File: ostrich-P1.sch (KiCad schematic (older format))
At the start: 25 parts

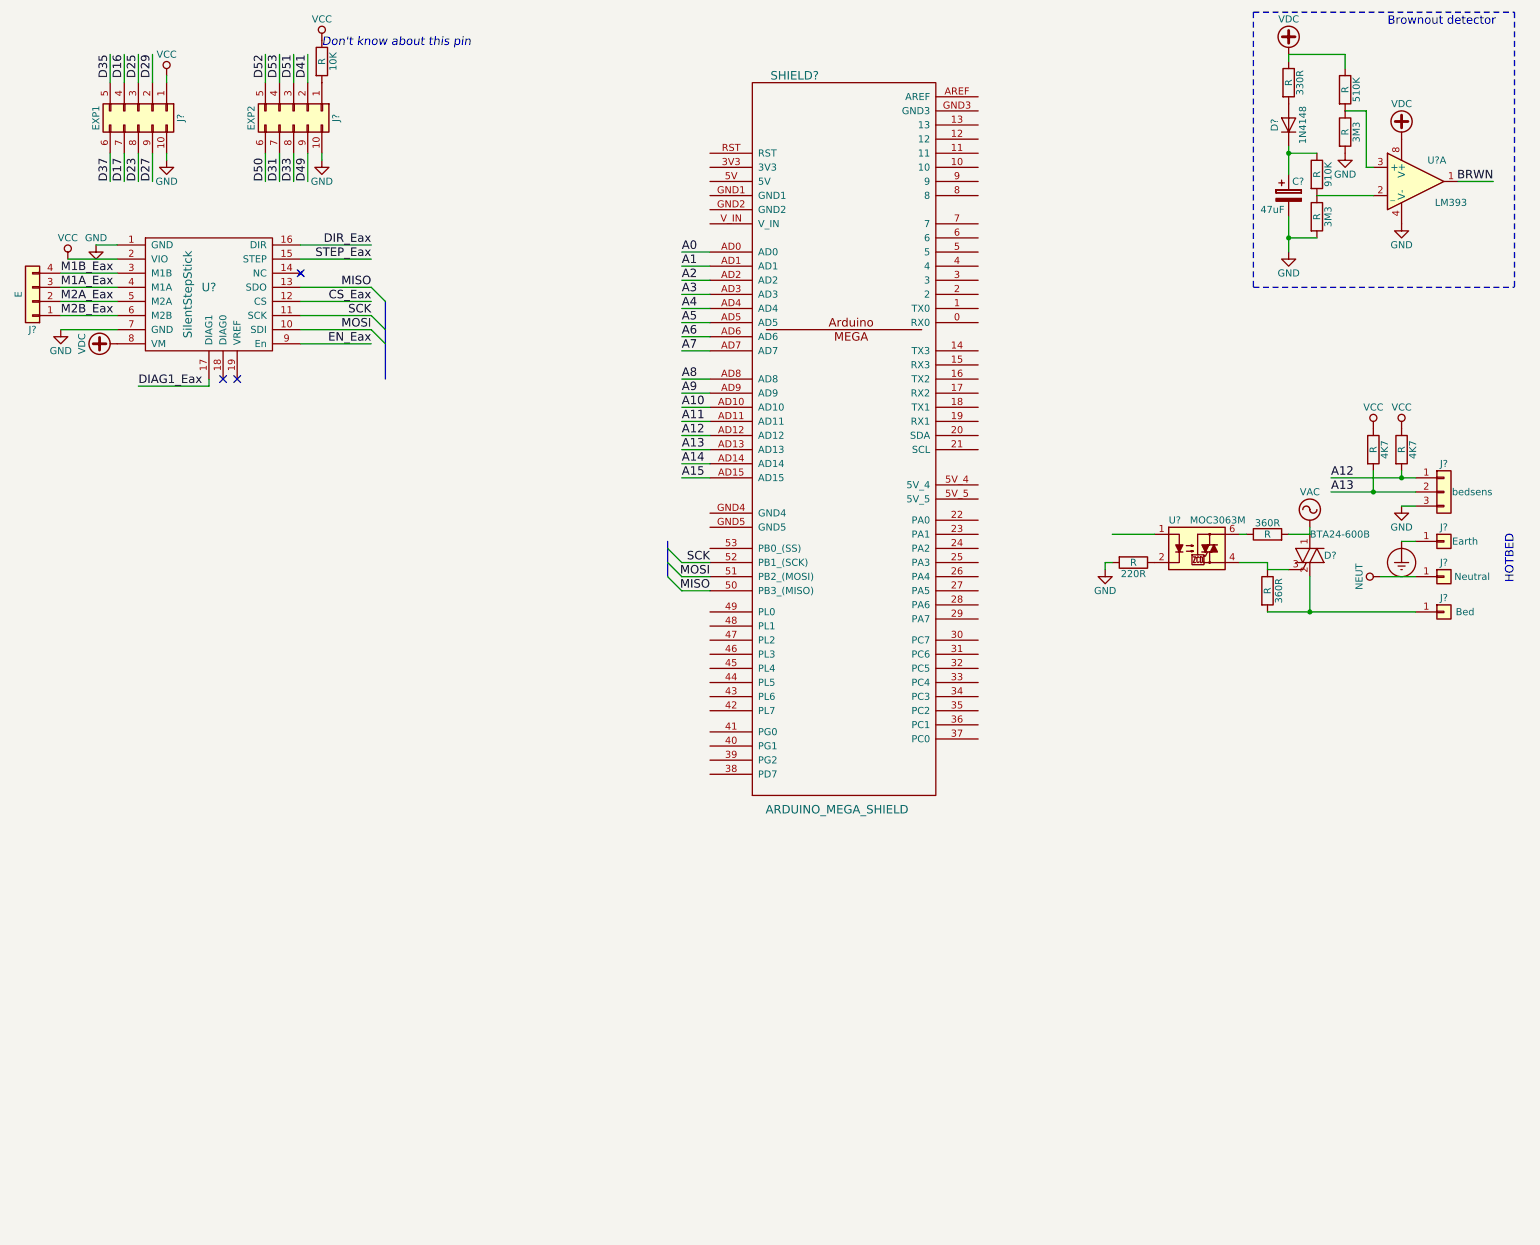
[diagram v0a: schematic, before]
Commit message: 3.3V reg and ESP12
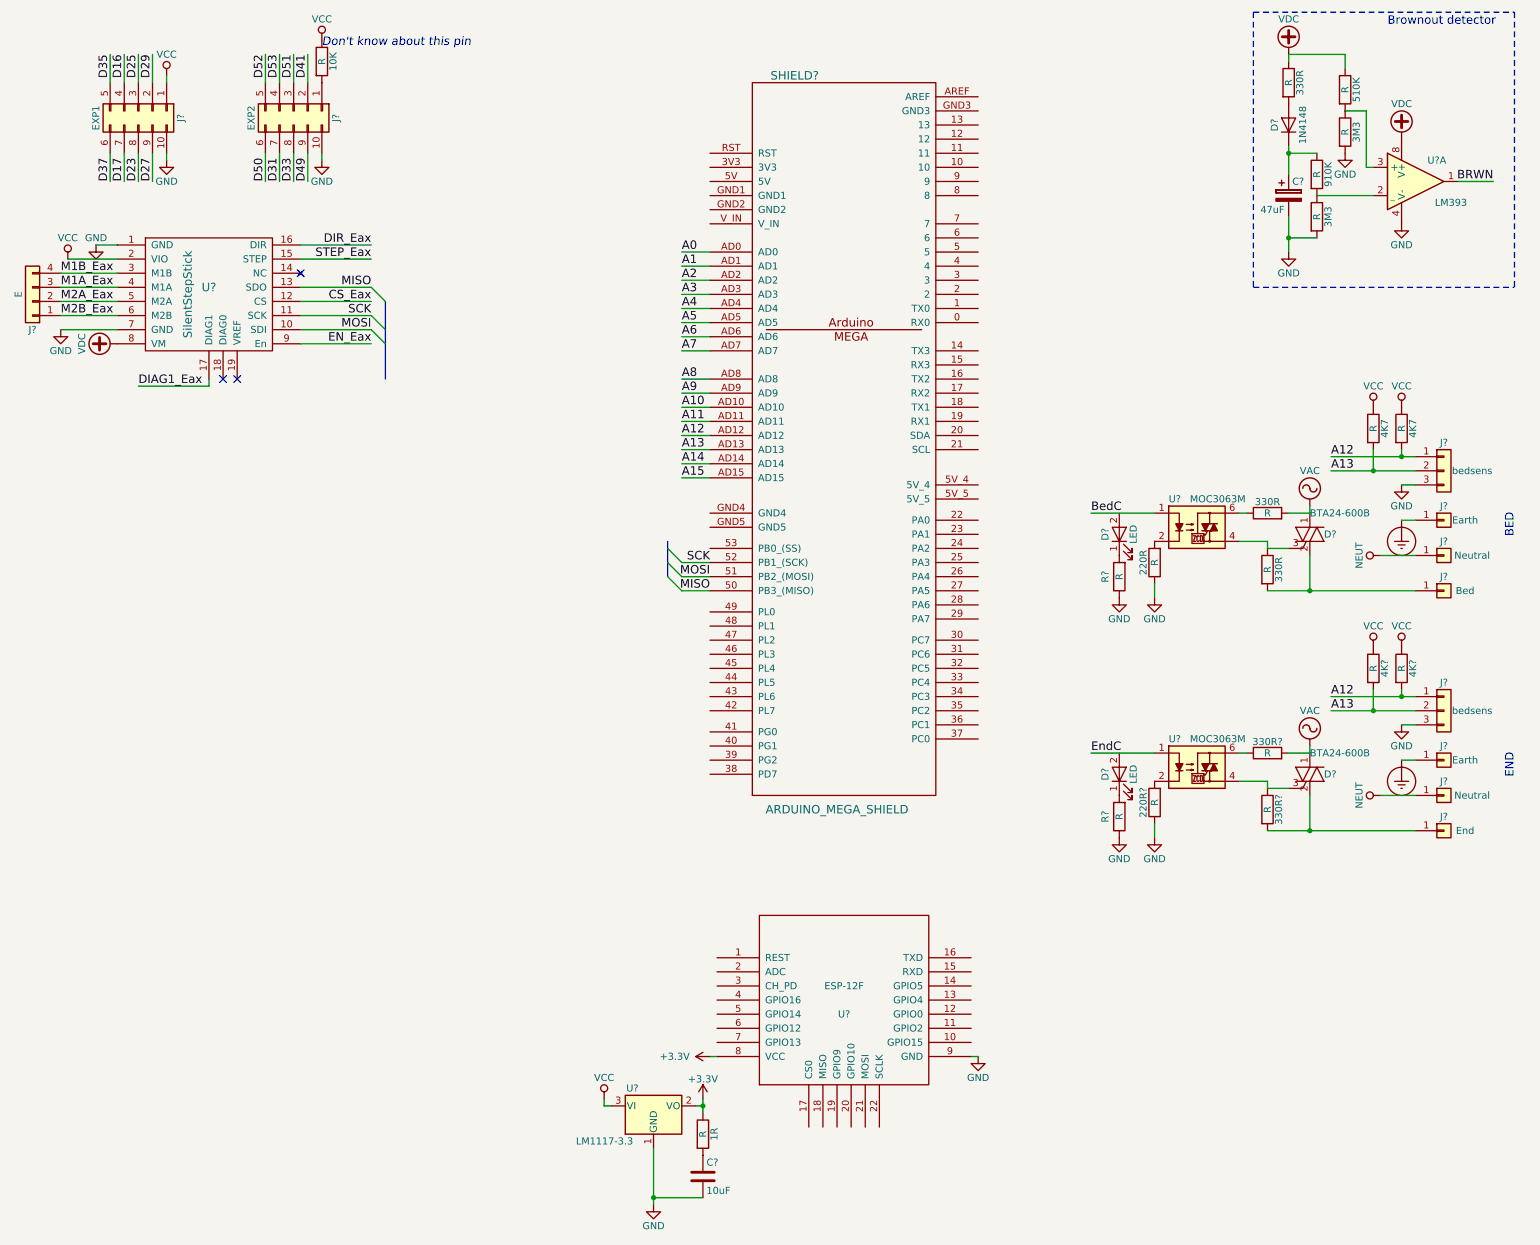
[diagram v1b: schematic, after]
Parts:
- added 1R, 220R?, 330R? (x2), 4K? (x2), R? (x2): R, symbol R
- added C?: 10uF, symbol C
- added D? (x2): LED, symbol LED
- added D?: BTA24-600B, symbol Q_TRIAC_AAG
- added J?: bedsens, symbol Conn_01x03
- added J?: Earth, symbol Conn_01x01
- added J?: Neutral, symbol Conn_01x01
- added J?: End, symbol Conn_01x01
- added U?: MOC3063M, symbol MOC3063M
- added U?: LM1117-3.3, symbol LM1117-3.3
- added U?: ESP-12F, symbol ESP-12F
- renumbered 360R to 330R
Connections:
- net A12: now also 4K?.2, J?.1 (Pin_1)
- net A13: now also 4K?.2, J?.2 (Pin_2)
- net Earth_Protective: now also J?.1 (Pin_1)
- net GND: now also 220R.1, 220R?.1, C?.2, J?.3 (Pin_3), R?.1, R?.1, U?.1 (GND), U?.9 (GND); no longer 220R.2
- net NEUT: now also J?.1 (Pin_1)
- net VAC: now also 330R?.2, D?.1 (A1)
- net VCC: now also 4K?.1, 4K?.1, U?.3 (VI)
- net BedC: now reaches U?.1
- net at U?.2: now also 220R.2; no longer 220R.1
- new net: D?.1 (K), R?.2 (x2)
- new net: 330R?.2, D?.2 (A2), J?.1 (Pin_1)
- new net: 330R?.1, D?.3 (G), U?.4
- new net: 220R?.2, U?.2
- new net: 330R?.1, U?.6
- new net: 1R.2, C?.1
- new net +3V3: 1R.1, U?.2 (VO), U?.8 (VCC)
- new net EndC: U?.1
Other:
- note added: "BED"
- note added: "END"
- note removed: "HOTBED"
- moved on the sheet: 220R, 330R, 4K7, D?, J?, U?
